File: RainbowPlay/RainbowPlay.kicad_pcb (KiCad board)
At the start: 4 copper layers, 92.3 x 60 mm, 64 parts, among them J1 GPIO_CONNECTOR, J2 Conn_01x06_Male, J3 Conn_01x04_Male, J4 Conn_01x02_Male, J5 Conn_01x02_Male, Q1 BSS138, Q2 BSS138, Q3 BSS138, Q4 BSS138, SW1 SW_SPST, U1 TPA2001D2, U2 SN74LVC1G32DBVRG4

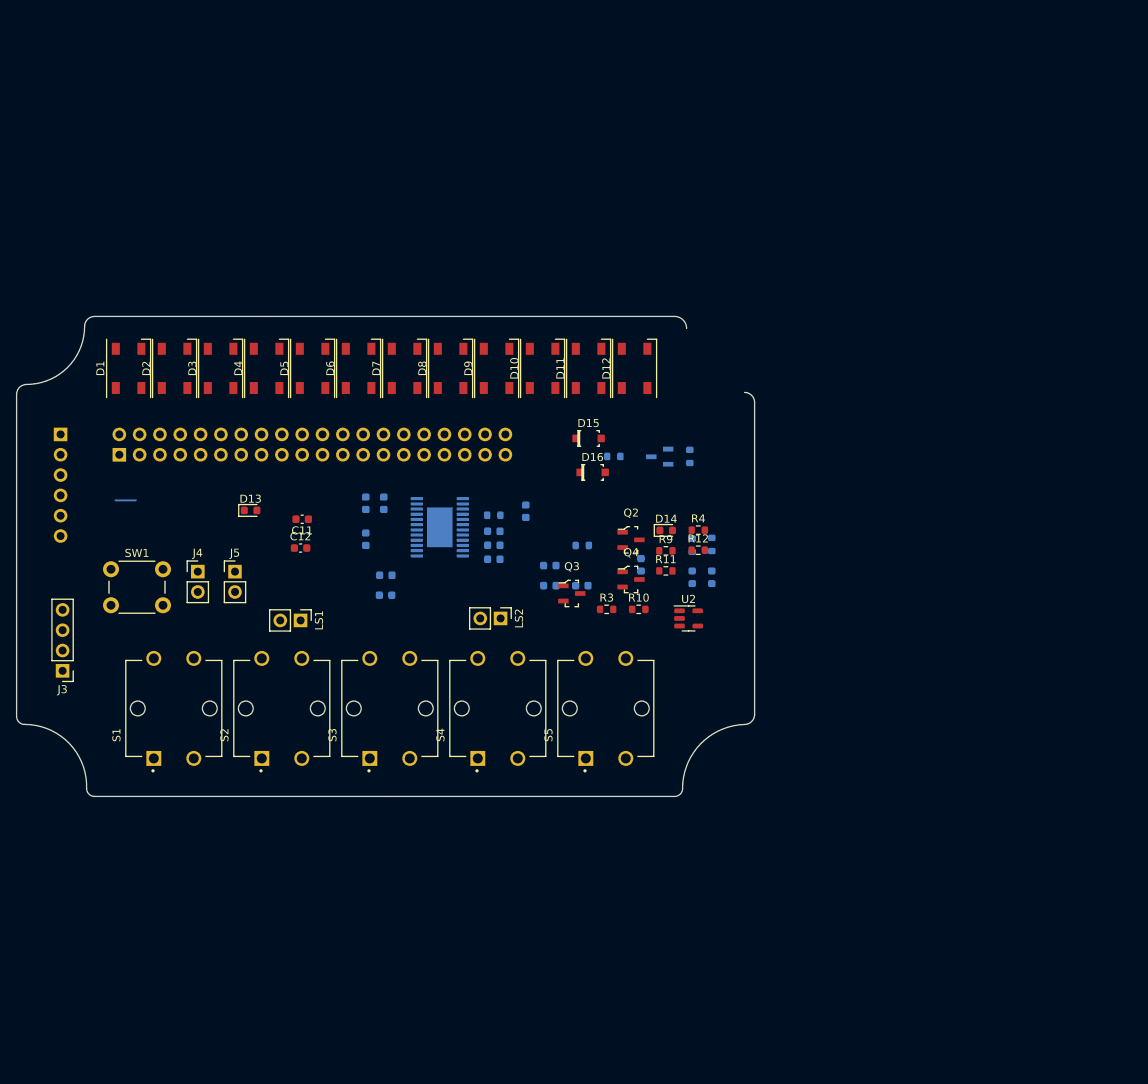
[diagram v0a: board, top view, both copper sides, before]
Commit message: Dev
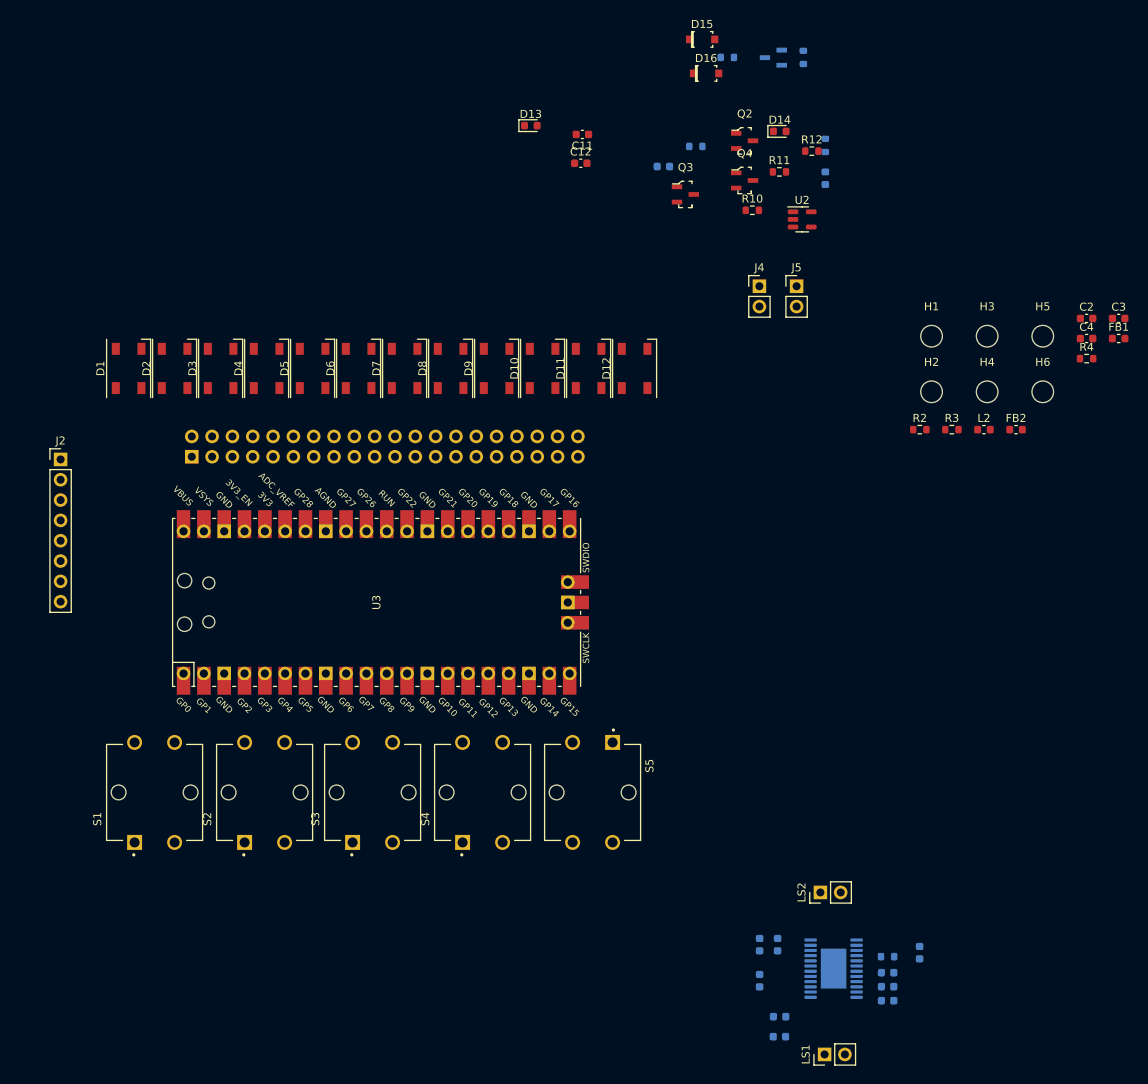
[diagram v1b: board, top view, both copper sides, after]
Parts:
- removed C6: 10uF, Capacitor_SMD:C_0603_1608Metric
- removed J3: Conn_01x04_Male, Connector_PinHeader_2.54mm:PinHeader_1x04_P2.54mm_Vertical
- removed R9: 200k, Resistor_SMD:R_0603_1608Metric
- removed SW1: SW_SPST, Button_Switch_THT:SW_PUSH_6mm
- added C2: 1.5uF, Capacitor_SMD:C_0603_1608Metric, F.Cu at (245.0, 63.3)
- added FB1: FerriteBead_Small, Inductor_SMD:L_0603_1608Metric, F.Cu at (249.0, 65.8)
- added FB2: FerriteBead_Small, Inductor_SMD:L_0603_1608Metric, F.Cu at (236.2, 77.2)
- added H1: MountingHole, MountingHole:MountingHole_2.7mm, F.Cu at (225.7, 65.5)
- added H2: MountingHole, MountingHole:MountingHole_2.7mm, F.Cu at (225.7, 72.5)
- added H3: MountingHole, MountingHole:MountingHole_2.7mm, F.Cu at (232.6, 65.5)
- added H4: MountingHole, MountingHole:MountingHole_2.7mm, F.Cu at (232.6, 72.5)
- added H5: MountingHole, MountingHole:MountingHole_2.7mm, F.Cu at (239.6, 65.5)
- added H6: MountingHole, MountingHole:MountingHole_2.7mm, F.Cu at (239.6, 72.5)
- added U3: Pico, MCU_RaspberryPi_and_Boards:RPi_Pico_SMD_TH, F.Cu at (156.3, 98.8)
- C3: value 1.5uF -> 10uF; moved to F.Cu
- C4, L2: moved to F.Cu
- J2: value Conn_01x06_Male -> Conn_01x08_Male; footprint Connector_PinHeader_2.54mm:PinHeader_1x06_P2.54mm_Vertical -> Connector_PinHeader_2.54mm:PinHeader_1x08_P2.54mm_Vertical; moved to F.Cu
- R2: value 5R -> 10k; moved to F.Cu
- R3: value 10k -> 5R
- moved LS1 85.0 mm to (212.3, 155.3), turned to 90 degrees
- moved J4 78.7 mm to (204.1, 59.3)
- moved J5 78.7 mm to (208.8, 59.3)
- moved C3 78.6 mm to (249.0, 63.3)
- moved C10 73.9 mm to (206.4, 141.6)
- moved C13 73.9 mm to (220.2, 145.1)
- moved C14 73.9 mm to (220.2, 148.6)
- moved C15 73.9 mm to (220.2, 146.8)
- moved C16 73.9 mm to (224.2, 142.6)
- moved C7 73.9 mm to (206.7, 150.6)
- moved C8 73.9 mm to (204.2, 141.6)
- moved C9 73.9 mm to (204.2, 146.1)
- moved R7 73.9 mm to (220.2, 143.1)
- moved U1 73.9 mm to (213.4, 144.6)
- moved C1 73.9 mm to (206.6, 153.1)
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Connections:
- C10 pad 1: GND -> GND1
- C11 pad 1: GND -> GND1
- C11 pad 2: +5V -> +5VA
- C12 pad 1: +5V -> +5VA
- C12 pad 2: GND -> GND1
- C13 pad 1: +5V -> +5VA
- C13 pad 2: GND -> GND1
- C14 pad 1: GND -> GND1
- C15 pad 1: GND -> GND1
- C15 pad 2: +5V -> +5VA
- C16 pad 1: GND -> GND1
- C16 pad 2: +5V -> +5VA
- C3 pad 1: GNDA -> /AUD_L+
- C3 pad 2: Net-(C3-Pad2) -> Net-(C2-Pad1)
- C4 pad 1: /AUD_L+ -> /AUD_L-
- C4 pad 2: Net-(C3-Pad2) -> GNDA
- C8 pad 1: +5V -> +5VA
- C8 pad 2: GND -> GND1
- C9 pad 1: +5V -> +5VA
- D1 pad 1: GND -> GND1
- D10 pad 1: GND -> GND1
- D11 pad 1: GND -> GND1
- D12 pad 1: GND -> GND1
- D12 pad 4: (no net) -> unconnected-(D12-Pad4)
- D2 pad 1: GND -> GND1
- D3 pad 1: GND -> GND1
- D4 pad 1: GND -> GND1
- D5 pad 1: GND -> GND1
- D6 pad 1: GND -> GND1
- D7 pad 1: GND -> GND1
- D8 pad 1: GND -> GND1
- D9 pad 1: GND -> GND1
- J1 pad 11: (no net) -> /BTN_A
- J1 pad 12: /LED -> unconnected-(J1-Pad12)
- J1 pad 13: (no net) -> /BTN_B
- J1 pad 14: (no net) -> unconnected-(J1-Pad14)
- J1 pad 15: (no net) -> unconnected-(J1-Pad15)
- J1 pad 16: /BTN_A -> unconnected-(J1-Pad16)
- J1 pad 17: (no net) -> unconnected-(J1-Pad17)
- J1 pad 18: /BTN_B -> unconnected-(J1-Pad18)
- J1 pad 19: (no net) -> unconnected-(J1-Pad19)
- J1 pad 21: (no net) -> unconnected-(J1-Pad21)
- J1 pad 22: (no net) -> unconnected-(J1-Pad22)
- J1 pad 23: (no net) -> unconnected-(J1-Pad23)
- J1 pad 24: (no net) -> unconnected-(J1-Pad24)
- J1 pad 25: (no net) -> unconnected-(J1-Pad25)
- J1 pad 26: (no net) -> unconnected-(J1-Pad26)
- J1 pad 3: (no net) -> unconnected-(J1-Pad3)
- J1 pad 30: (no net) -> unconnected-(J1-Pad30)
- J1 pad 34: (no net) -> unconnected-(J1-Pad34)
- J1 pad 39: (no net) -> unconnected-(J1-Pad39)
- J1 pad 40: (no net) -> /PWR_BTN
- J1 pad 5: (no net) -> /WAKE_ON_GPIO
- J1 pad 6: (no net) -> unconnected-(J1-Pad6)
- J1 pad 7: (no net) -> /LO_BATT
- J1 pad 9: (no net) -> unconnected-(J1-Pad9)
- J2 pad 2: (no net) -> unconnected-(J2-Pad2)
- J2 pad 3: (no net) -> unconnected-(J2-Pad3)
- J2 pad 5: /PWR_EN -> unconnected-(J2-Pad5)
- J2 pad 6: /Vs -> unconnected-(J2-Pad6)
- L2 pad 2: Net-(C3-Pad2) -> Net-(C2-Pad1)
- Q1 pad 2: /LED -> /NEO
- Q2 pad 1: +3V3 -> /AWAKE_SIG
- Q2 pad 2: /AWAKE_SIG -> GND
- Q2 pad 3: Net-(Q2-Pad3) -> GND1
- Q3 pad 2: GND -> GND1
- Q4 pad 2: GND -> GND1
- R11 pad 1: GND -> GND1
- R12 pad 1: GND -> GND1
- R2 pad 1: Net-(L2-Pad1) -> /PWR_BTN
- R2 pad 2: /PWM_AUDIO_L -> +3V3
- R3 pad 1: GND -> Net-(L2-Pad1)
- R3 pad 2: /AWAKE_SIG -> /PWM_AUDIO_L
- R4 pad 1: Net-(R4-Pad1) -> /AWAKE_SIG
- R4 pad 2: /Vs -> GND
- R5 pad 1: /LED -> /NEO
- R7 pad 1: GND -> GND1
- R8 pad 1: GND -> GND1
- U1 pad 1: GND -> GND1
- U1 pad 10: +5V -> +5VA
- U1 pad 12: GND -> GND1
- U1 pad 13: GND -> GND1
- U1 pad 16: +5V -> +5VA
- U1 pad 19: +5V -> +5VA
- U1 pad 21: +5V -> +5VA
- U1 pad 24: GND -> GND1
- U1 pad 4: +5V -> +5VA
- U1 pad 9: +5V -> +5VA
- U2 pad 1: Net-(Q2-Pad3) -> /AWAKE_SIG
- U2 pad 2: Net-(R4-Pad1) -> /PWR_BTN
- U2 pad 4: /PWR_EN -> Net-(Q5-Pad1)
- U2 pad 5: /Vs -> +3V3
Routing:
- net +5V: track 2.54 -> 0.00 mm
- removed copper zone on In2.Cu, net GND
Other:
- board outline removed
- net class Default removed
